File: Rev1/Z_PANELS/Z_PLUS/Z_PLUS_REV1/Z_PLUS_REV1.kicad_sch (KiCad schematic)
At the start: 1 part, among them J1 F3311A7H121014E200

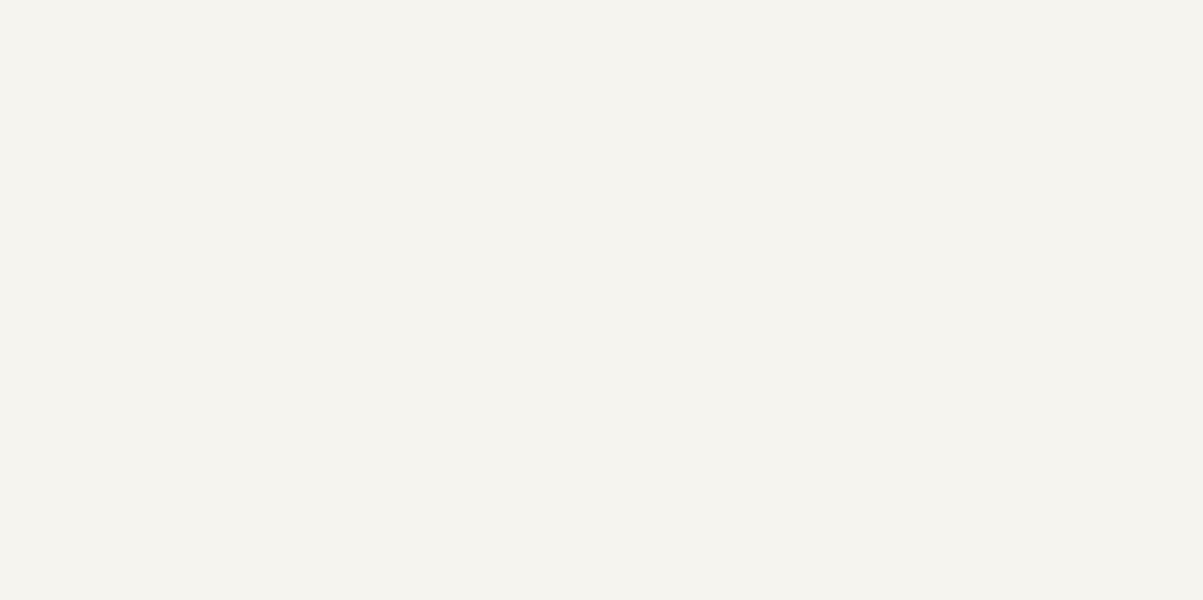
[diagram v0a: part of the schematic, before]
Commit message: fixed bugs and finished Z plus
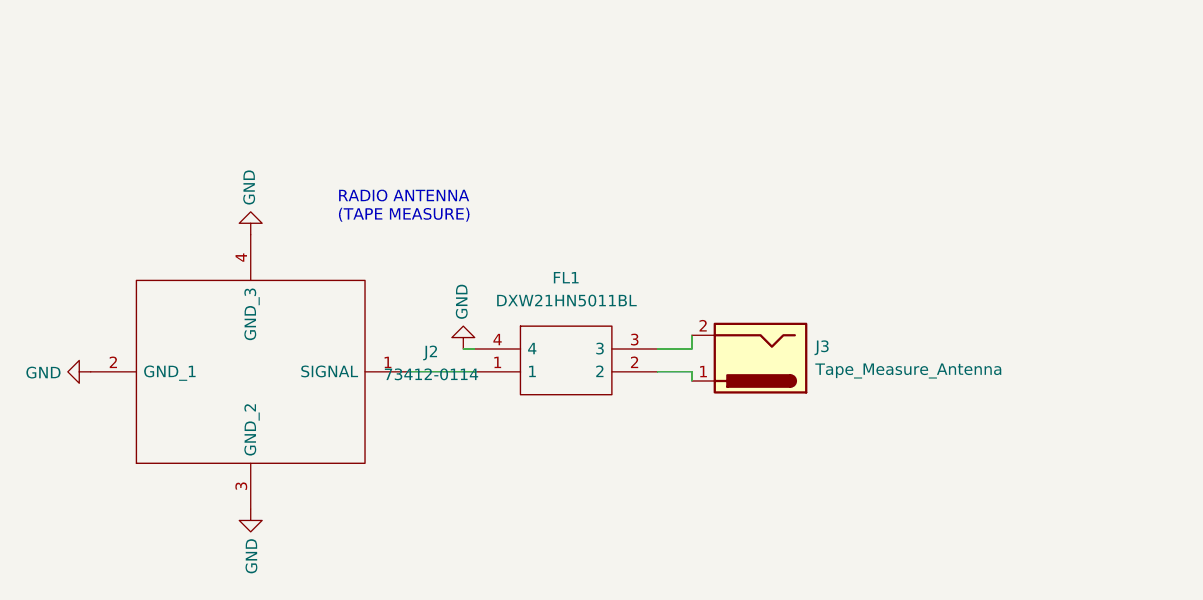
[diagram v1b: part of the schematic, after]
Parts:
- added FL1: DXW21HN5011BL, DXW21HN5011BL, symbol AA_AUTO_LOADER:DXW21HN5011BL
- added J2: 73412-0114, 73412-0110, symbol AA_AUTO_LOADER:73412-0114
- added J3: Tape_Measure_Antenna, Audio_Module:Radio_antenna, symbol Connector:Tape_measure_antenna
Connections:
- net GND: now also FL1.4, J2.2 (GND_1), J2.3 (GND_2), J2.4 (GND_3)
- new net: FL1.1, J2.1 (SIGNAL)
- new net: FL1.2, J3.1
- new net: FL1.3, J3.2
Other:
- note added: "RADIO ANTENNA (TAPE MEASURE)"
